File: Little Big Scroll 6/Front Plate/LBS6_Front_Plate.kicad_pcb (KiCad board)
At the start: 2 copper layers, 57.2 x 85 mm, 13 parts, among them SW1 SW_Push, SW2 SW_Push, SW3 SW_Push, SW4 SW_Push, SW5 SW_Push, SW6 SW_Push, SW7 Rotary_Encoder_Switch

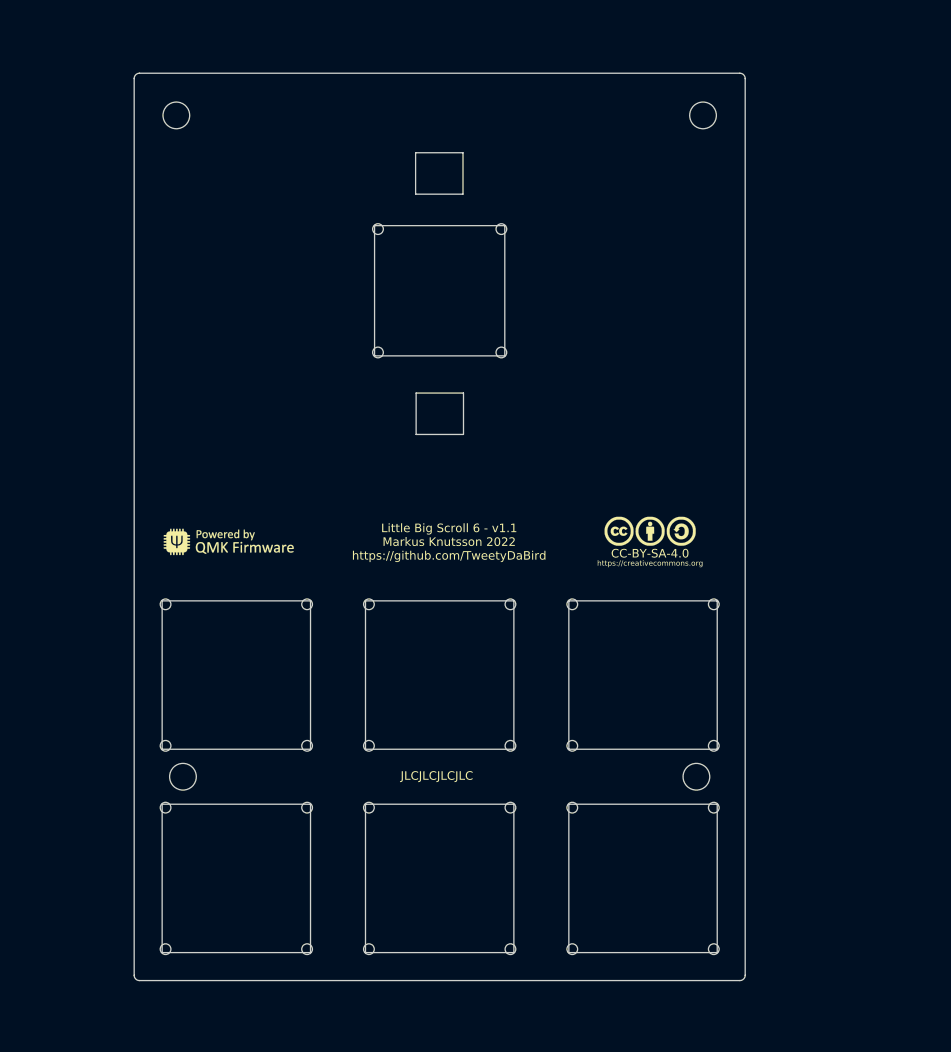
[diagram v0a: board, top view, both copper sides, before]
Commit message: LSB6 1.01
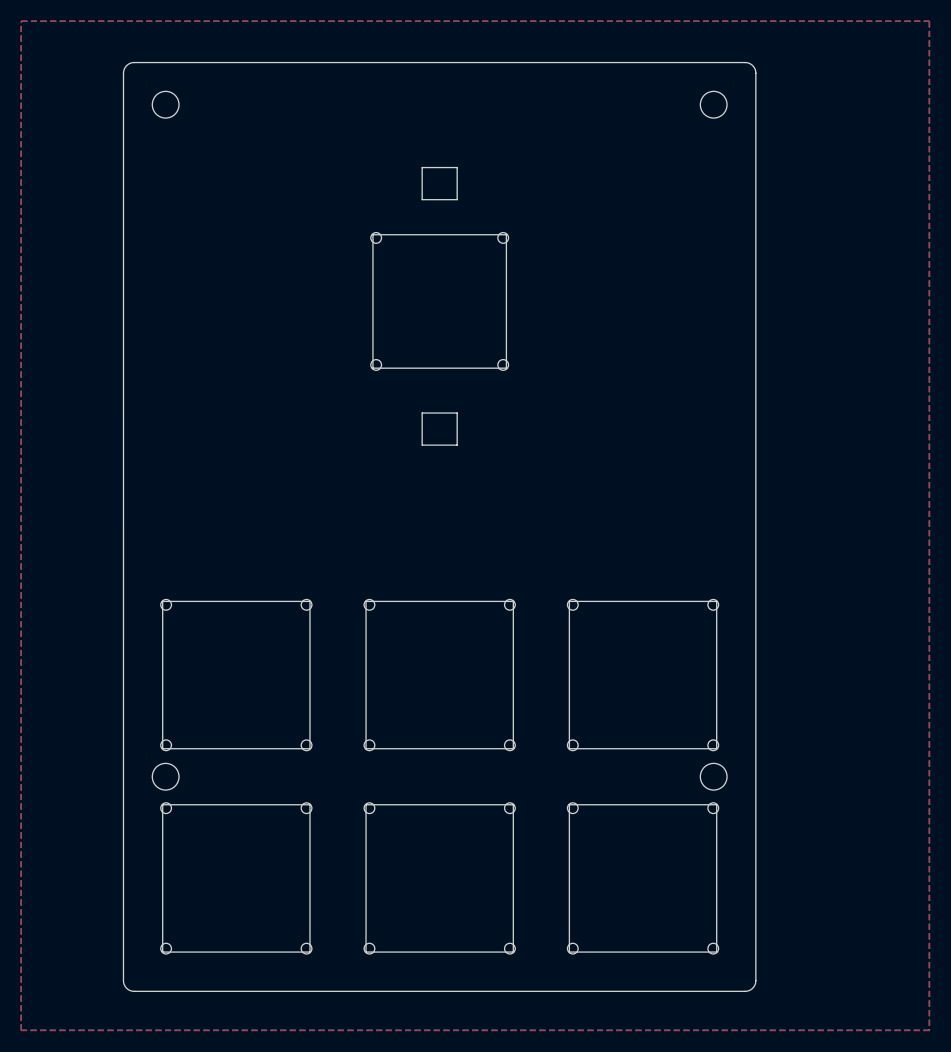
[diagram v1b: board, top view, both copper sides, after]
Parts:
- removed Lic1: CC-BY-SA-4.0, CC_Licensing:CC_BY_SA_40
- removed Logo1: QMK_Logo, QMK Logo:Powered_by_QMK
- ENC1: renamed from SW7; value Rotary_Encoder_Switch -> Rotary_Encoder_Click; footprint Tweety keyswitches:Plate_Encoder -> Keyboard Switches & Encoders:Encoder_Plate_Placeholder
- H1, H2, H3, H4: value Hole_PCB_M2-Spacer -> Spacer_Plate; footprint Tweety keyswitches:Plate_Hole -> Keyboard Switches & Encoders:Spacer Plate hole
- SW1, SW2, SW3, SW4, SW5, SW6: footprint Tweety keyswitches:Cherry_MX_Plate_Placeholder -> Keyboard Switches & Encoders:SW_MX_Plate_Placeholder
- moved H1 1.62 mm to (84.6, 112.7)
- moved H2 1.62 mm to (135.9, 112.7)
- moved H3 1.41 mm to (135.9, 49.7)
- moved H4 1.41 mm to (84.6, 49.7)
- moved ENC1 1.00 mm to (110.3, 68.2)
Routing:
- added copper zone on B.Cu, net (none)
- added copper zone on F.Cu, net (none)
- added copper zone on B.Cu, net GND
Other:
- board size 57.2 x 85 mm -> 59.2 x 87 mm
- board text removed: "JLCJLCJLCJLC"
- board text removed: "Little Big Scroll 6 - v1.1 Markus Knutsson 2022 https://github.com/TweetyDaBird"
